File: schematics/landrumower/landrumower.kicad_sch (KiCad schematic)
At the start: 26 parts, among them J1 UART, J10 Lift, J11 MotorLeft, J12 Conn_01x06_Female, J13 Conn_01x06_Female, J14 Rain, J15 MotorMow, J16 Conn_01x06_Female, J17 Conn_01x06_Female, J18 StopButton, J19 ReserveGPIO, J2 I2C0, J20 ResrveGPIO/ADC0, J21 ReserveGPIO/ADC1, J3 Power, J4 I2C1, J5 BumperX, J6 MotorRight, J7 Conn_01x06_Female, J8 Conn_01x06_Female, J9 BumperY, U1 Pico

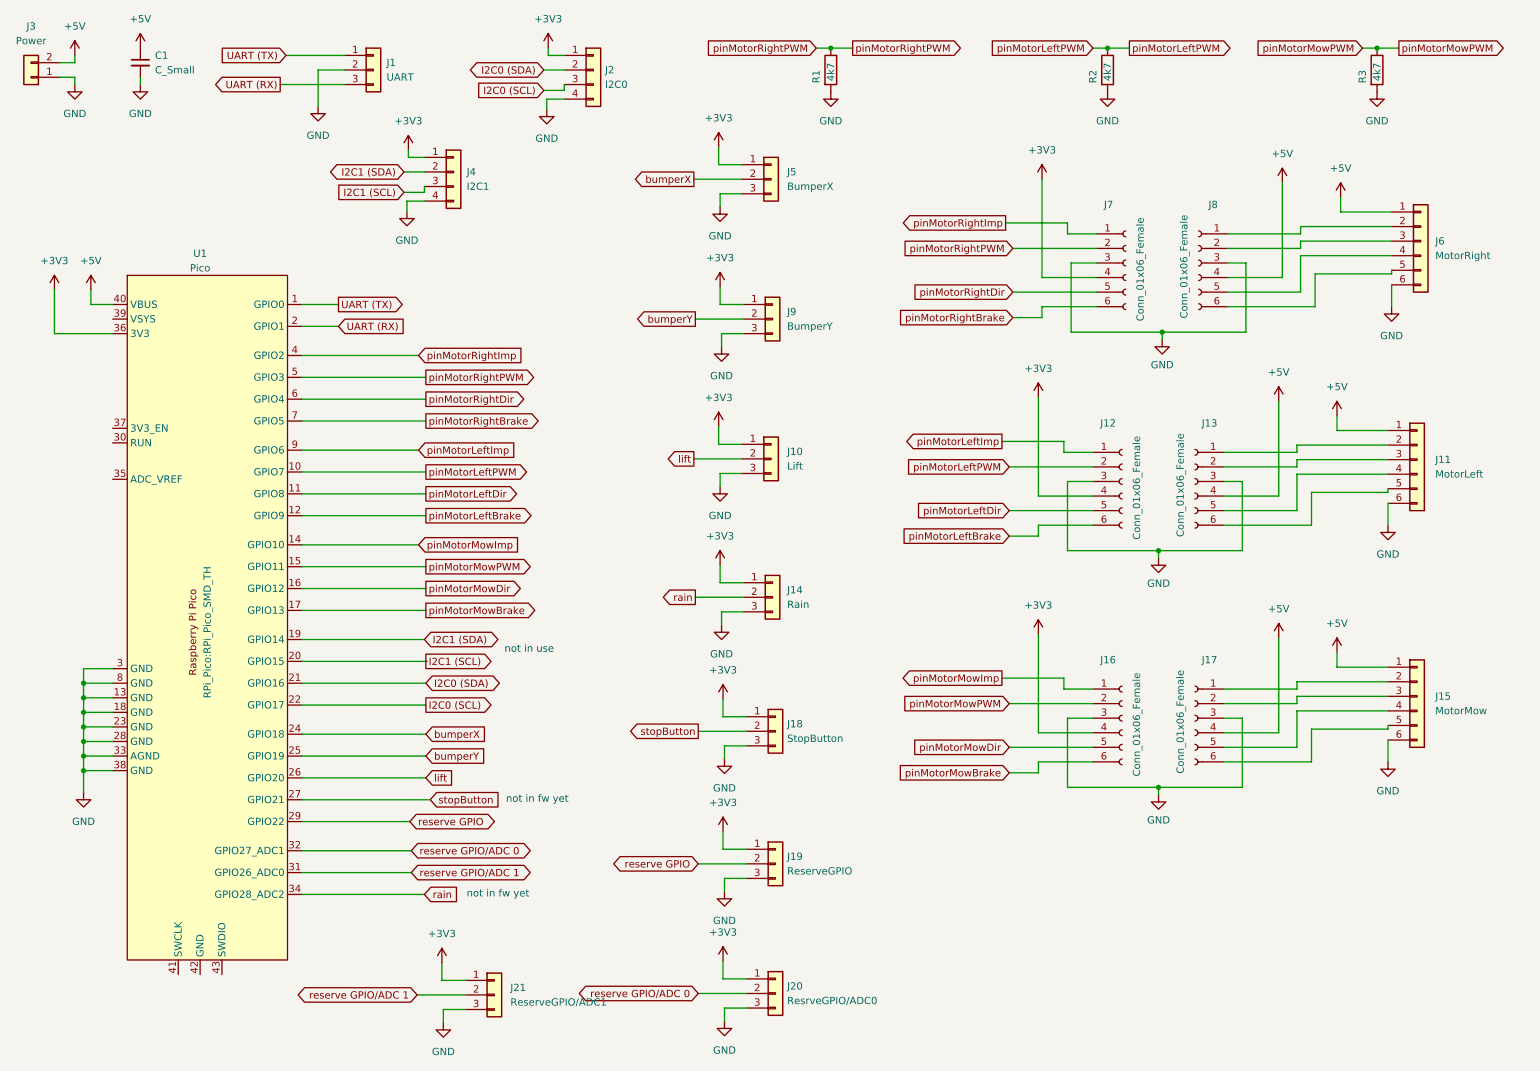
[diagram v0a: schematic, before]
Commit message: Update schematics for landrumower pcb
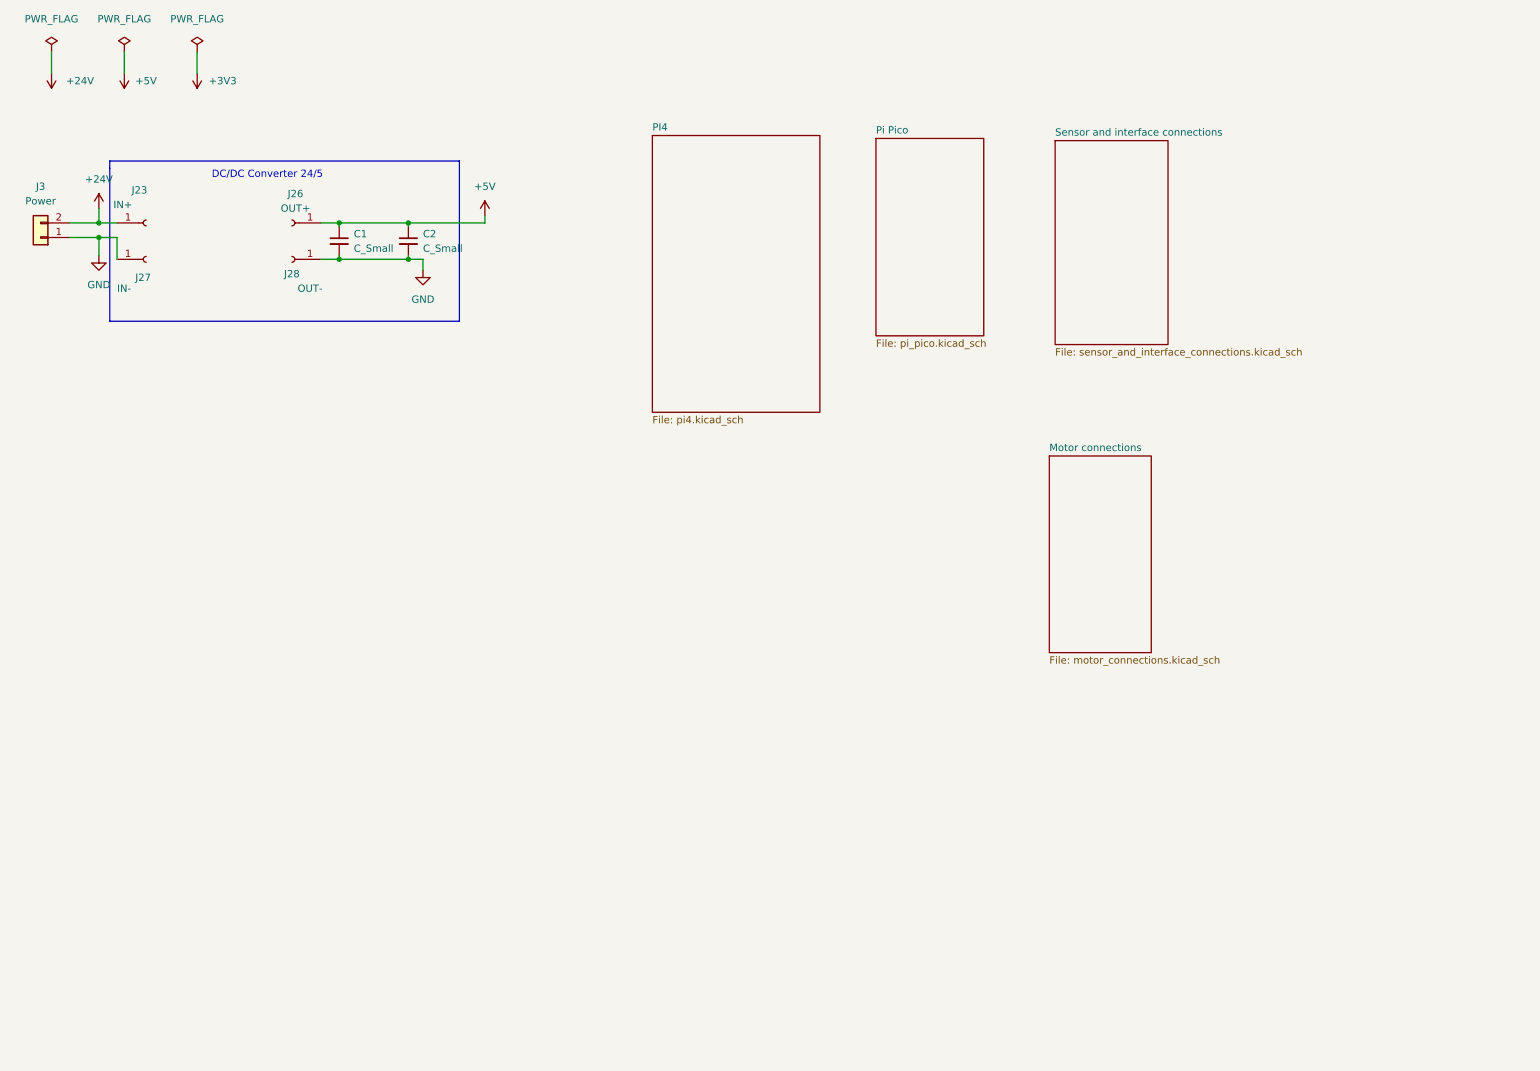
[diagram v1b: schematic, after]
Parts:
- removed J1: UART, Connector_JST:JST_EH_B3B-EH-A_1x03_P2.50mm_Vertical, symbol Connector_Generic:Conn_01x03
- removed J10: Lift, Connector_JST:JST_EH_B3B-EH-A_1x03_P2.50mm_Vertical, symbol Connector_Generic:Conn_01x03
- removed J11: MotorLeft, Connector_JST:JST_EH_B6B-EH-A_1x06_P2.50mm_Vertical, symbol Connector_Generic:Conn_01x06
- removed J12, J13, J16, J17, J7, J8: Conn_01x06_Female, Connector_PinSocket_2.54mm:PinSocket_1x06_P2.54mm_Vertical, symbol Connector:Conn_01x06_Female
- removed J14: Rain, Connector_JST:JST_EH_B3B-EH-A_1x03_P2.50mm_Vertical, symbol Connector_Generic:Conn_01x03
- removed J15: MotorMow, Connector_JST:JST_EH_B6B-EH-A_1x06_P2.50mm_Vertical, symbol Connector_Generic:Conn_01x06
- removed J18: StopButton, Connector_JST:JST_EH_B3B-EH-A_1x03_P2.50mm_Vertical, symbol Connector_Generic:Conn_01x03
- removed J19: ReserveGPIO, Connector_JST:JST_EH_B3B-EH-A_1x03_P2.50mm_Vertical, symbol Connector_Generic:Conn_01x03
- removed J2: I2C0, Connector_JST:JST_EH_B4B-EH-A_1x04_P2.50mm_Vertical, symbol Connector_Generic:Conn_01x04
- removed J20: ResrveGPIO/ADC0, Connector_JST:JST_EH_B3B-EH-A_1x03_P2.50mm_Vertical, symbol Connector_Generic:Conn_01x03
- removed J21: ReserveGPIO/ADC1, Connector_JST:JST_EH_B3B-EH-A_1x03_P2.50mm_Vertical, symbol Connector_Generic:Conn_01x03
- removed J4: I2C1, Connector_JST:JST_EH_B4B-EH-A_1x04_P2.50mm_Vertical, symbol Connector_Generic:Conn_01x04
- removed J5: BumperX, Connector_JST:JST_EH_B3B-EH-A_1x03_P2.50mm_Vertical, symbol Connector_Generic:Conn_01x03
- removed J6: MotorRight, Connector_JST:JST_EH_B6B-EH-A_1x06_P2.50mm_Vertical, symbol Connector_Generic:Conn_01x06
- removed J9: BumperY, Connector_JST:JST_EH_B3B-EH-A_1x03_P2.50mm_Vertical, symbol Connector_Generic:Conn_01x03
- removed R1, R2, R3: 4k7, Resistor_SMD:R_0805_2012Metric_Pad1.20x1.40mm_HandSolder, symbol Device:R
- removed U1: Pico, RPi_Pico:RPi_Pico_SMD_TH, symbol MCU_RaspberryPi_and_Boards:Pico
- added C2: C_Small, Capacitor_SMD:C_0805_2012Metric_Pad1.18x1.45mm_HandSolder, symbol Device:C_Small
- added J23: IN+, Connector_PinSocket_2.54mm:PinSocket_1x01_P2.54mm_Vertical, symbol Connector:Conn_01x01_Female
- added J26: OUT+, Connector_PinSocket_2.54mm:PinSocket_1x01_P2.54mm_Vertical, symbol Connector:Conn_01x01_Female
- added J27: IN-, Connector_PinSocket_2.54mm:PinSocket_1x01_P2.54mm_Vertical, symbol Connector:Conn_01x01_Female
- added J28: OUT-, Connector_PinSocket_2.54mm:PinSocket_1x01_P2.54mm_Vertical, symbol Connector:Conn_01x01_Female
- J3: footprint Connector_JST:JST_EH_B2B-EH-A_1x02_P2.50mm_Vertical -> TerminalBlock:TerminalBlock_Altech_AK300-2_P5.00mm
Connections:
- net +5V: now also C2.1, J26.1 (Pin_1); no longer J3.2 (Pin_2)
- net GND: now also C2.2, J27.1 (Pin_1), J28.1 (Pin_1)
- new net +24V: J23.1 (Pin_1), J3.2 (Pin_2)
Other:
- added sheet Motor connections (motor_connections.kicad_sch)
- added sheet PI4 (pi4.kicad_sch)
- added sheet Pi Pico (pi_pico.kicad_sch)
- added sheet Sensor and interface connections (sensor_and_interface_connections.kicad_sch)
- note added: "DC/DC Converter 24/5"
- note removed: "not in fw yet"
- note removed: "not in use"
- moved on the sheet: C1, J3

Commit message: Update schematics
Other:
- title: Landrumower RPi Pico -> Landrumower
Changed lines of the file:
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@@
   (paper "A4")
   (title_block
-    (title "Landrumower RPi Pico")
+    (title "Landrumower")
     (rev "1.0")
   )

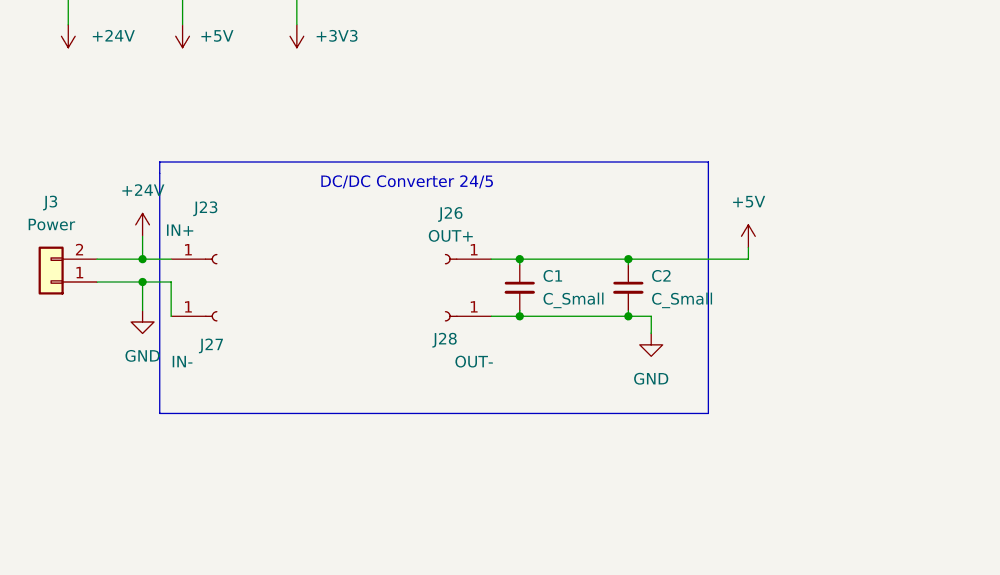
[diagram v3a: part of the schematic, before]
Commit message: changes in schematics
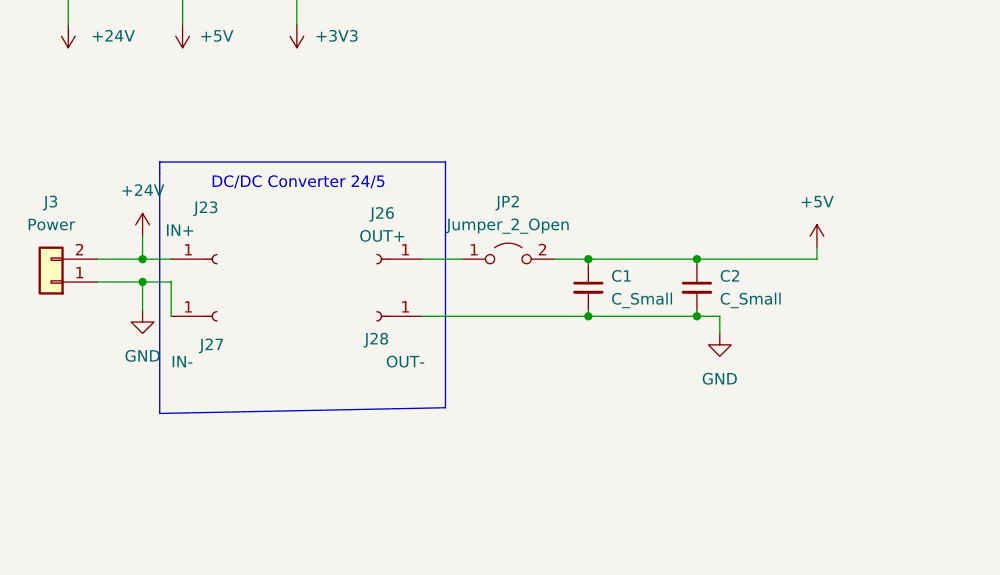
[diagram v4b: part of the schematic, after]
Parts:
- added JP2: Jumper_2_Open, Jumper:SolderJumper-2_P1.3mm_Open_Pad1.0x1.5mm, symbol Jumper:Jumper_2_Open
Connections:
- net +5V: now also JP2.2 (B); no longer J26.1 (Pin_1)
- new net: J26.1 (Pin_1), JP2.1 (A)
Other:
- moved on the sheet: C1, C2, J26, J28
